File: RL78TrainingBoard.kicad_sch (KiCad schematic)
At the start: 88 parts, among them J1 USB_B_Mini, J2 DSub9pin_Male, J3 Debugger, J4 OLED, Q1 AO3400A, Q2 NJL7502L, SW1 SW_A, SW2 SW_B, SW3 SW_C, SW4 SW_D, SW5 RESET_SW, SW6 USER_SW, U1 TBD62783A, U2 FT230XS, U3 ADM3202, U4 SC1602B, U5 RL78G13_64pin, U6 LM60, U7 YMZ294, U8 HT82V739, Y1 32.768kHz

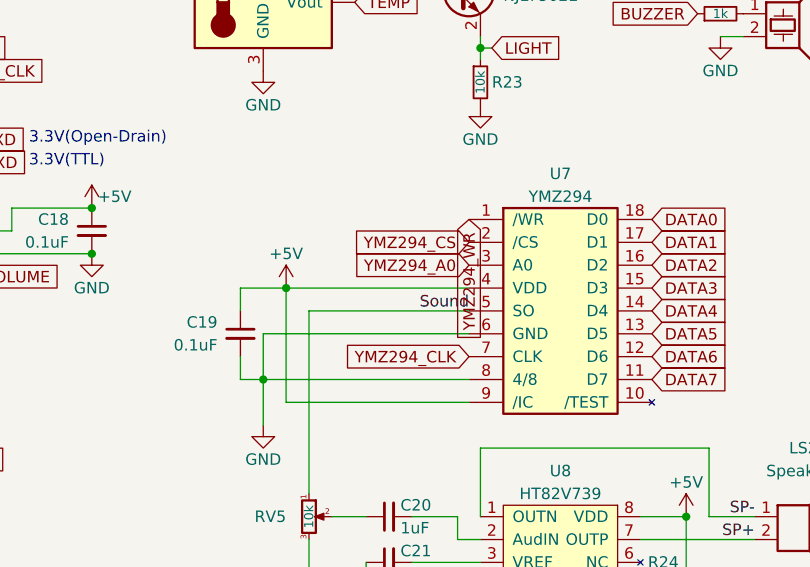
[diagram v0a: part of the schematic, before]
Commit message: 基板設計(部品仮配置)
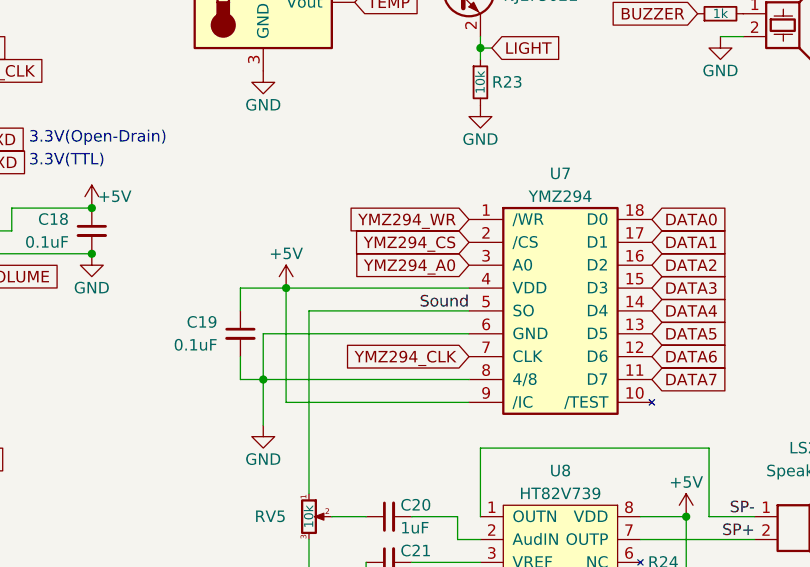
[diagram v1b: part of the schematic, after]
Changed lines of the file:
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@@
     )
   )
-  (global_label "YMZ294_WR" (shape input) (at 242.57 88.9 270) (fields_autoplaced)
+  (global_label "YMZ294_WR" (shape input) (at 242.57 88.9 180) (fields_autoplaced)
     (effects (font (size 1.27 1.27)) (justify right))
-    (property "シート間のリファレンス" "${INTERSHEET_REFS}" (id 0) (at 242.4906 102.3802 90)
+    (property "シート間のリファレンス" "${INTERSHEET_REFS}" (id 0) (at 229.0898 88.8206 0)
       (effects (font (size 1.27 1.27)) (justify right) hide)
     )
